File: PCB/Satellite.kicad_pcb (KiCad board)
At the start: 2 copper layers, 300 x 80 mm, 124 parts, among them SW1 SW_Push, SW10 SW_Push, SW11 SW_Push, SW12 SW_Push, SW13 SW_Push, SW14 SW_Push, SW15 SW_Push, SW16 SW_Push, SW17 SW_Push, SW18 SW_Push, SW19 SW_Push, SW2 SW_Push, SW20 SW_Push, SW21 SW_Push, SW22 SW_Push, SW23 SW_Push, SW24 SW_Push, SW25 SW_Push, SW26 SW_Push, SW27 SW_Push, SW28 SW_Push, SW29 SW_Push, SW3 SW_Push, SW30 SW_Push, SW31 SW_Push, SW32 SW_Push, SW33 SW_Push, SW34 SW_Push, SW35 SW_Push, SW36 SW_Push, SW37 SW_Push, SW38 SW_Push, SW39 SW_Push, SW4 SW_Push, SW40 SW_Push, SW41 SW_Push, SW42 SW_Push, SW43 SW_Push, SW44 SW_Push, SW45 SW_Push, SW46 SW_Push, SW47 SW_Push, SW48 SW_Push, SW5 SW_Push, SW6 SW_Push, SW7 SW_Push, SW8 SW_Push, SW9 SW_Push, Y1 16Mhz

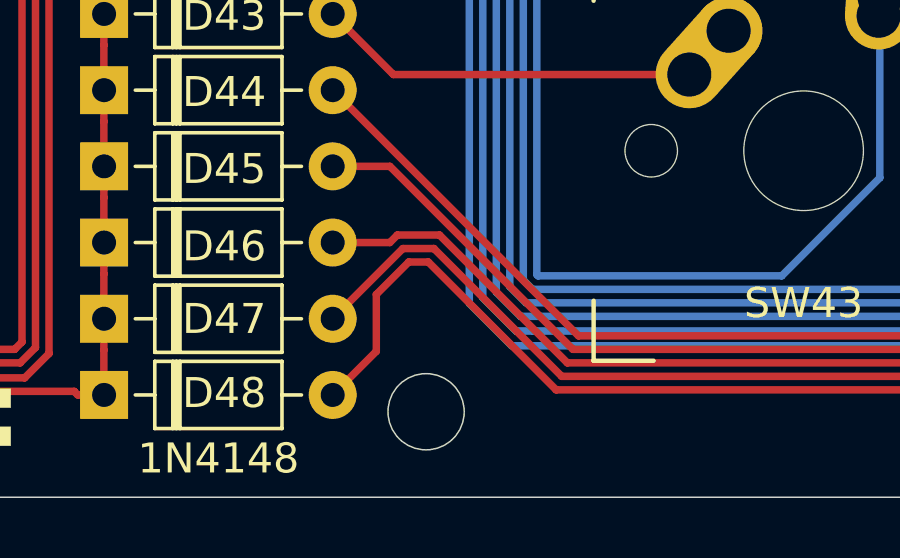
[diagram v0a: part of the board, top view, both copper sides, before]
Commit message: minor
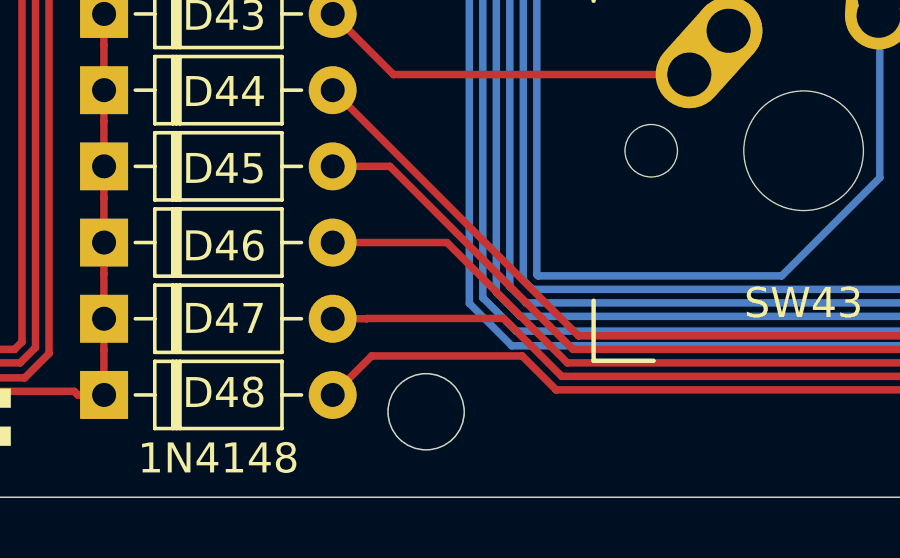
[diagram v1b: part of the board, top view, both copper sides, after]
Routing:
- net Net-(D48-Pad2): track 127.7 -> 124.0 mm
- net Net-(D47-Pad2): track 100.2 -> 98.2 mm
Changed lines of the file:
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@@
     (thickness 1.6)
     (drawings 28)
-    (tracks 936)
+    (tracks 934)
     (zones 0)
     (modules 124)
@@
   (segment (start 269.384018 101.479978) (end 269.38402 101.47998) (width 0.25) (layer F.Cu) (net 54))
   (segment (start 209.44716 101.479978) (end 269.384018 101.479978) (width 0.25) (layer F.Cu) (net 54))
-  (segment (start 205.187172 97.21999) (end 203.7796 97.21999) (width 0.25) (layer F.Cu) (net 54))
-  (segment (start 209.44716 101.479978) (end 205.187172 97.21999) (width 0.25) (layer F.Cu) (net 54))
-  (segment (start 203.52959 97.47) (end 201.626 97.47) (width 0.25) (layer F.Cu) (net 54))
-  (segment (start 203.7796 97.21999) (end 203.52959 97.47) (width 0.25) (layer F.Cu) (net 54))
+  (segment (start 205.43718 97.47) (end 209.44716 101.479978) (width 0.25) (layer F.Cu) (net 54))
+  (segment (start 201.626 97.47) (end 205.43718 97.47) (width 0.25) (layer F.Cu) (net 54))
   (segment (start 289.718 100.67598) (end 289.718 91.87) (width 0.25) (layer F.Cu) (net 55))
   (segment (start 288.46399 101.92999) (end 289.718 100.67598) (width 0.25) (layer F.Cu) (net 55))
-  (segment (start 201.626 100.01) (end 203.966 97.67) (width 0.25) (layer F.Cu) (net 55))
-  (segment (start 203.966 97.67) (end 205.000771 97.67) (width 0.25) (layer F.Cu) (net 55))
-  (segment (start 205.000771 97.67) (end 205.000771 97.670771) (width 0.25) (layer F.Cu) (net 55))
   (segment (start 288.463988 101.929988) (end 288.46399 101.92999) (width 0.25) (layer F.Cu) (net 55))
   (segment (start 209.259988 101.929988) (end 288.463988 101.929988) (width 0.25) (layer F.Cu) (net 55))
-  (segment (start 205.000771 97.670771) (end 209.259988 101.929988) (width 0.25) (layer F.Cu) (net 55))
+  (segment (start 202.75737 100.01) (end 202.76737 100) (width 0.25) (layer F.Cu) (net 55))
+  (segment (start 201.626 100.01) (end 202.75737 100.01) (width 0.25) (layer F.Cu) (net 55))
+  (segment (start 207.33 100) (end 209.259988 101.929988) (width 0.25) (layer F.Cu) (net 55))
+  (segment (start 202.76737 100) (end 207.33 100) (width 0.25) (layer F.Cu) (net 55))
   (segment (start 308.768 100.996) (end 308.768 91.87) (width 0.25) (layer F.Cu) (net 56))
   (segment (start 301.267002 102.38) (end 301.277002 102.39) (width 0.25) (layer F.Cu) (net 56))
   (segment (start 301.277002 102.39) (end 307.374 102.39) (width 0.25) (layer F.Cu) (net 56))
   (segment (start 307.374 102.39) (end 308.768 100.996) (width 0.25) (layer F.Cu) (net 56))
-  (segment (start 201.626 102.55) (end 203.08 101.096) (width 0.25) (layer F.Cu) (net 56))
-  (segment (start 203.08 99.2) (end 204.15999 98.12001) (width 0.25) (layer F.Cu) (net 56))
-  (segment (start 203.08 101.096) (end 203.08 99.2) (width 0.25) (layer F.Cu) (net 56))
-  (segment (start 204.15999 98.12001) (end 204.8136 98.12001) (width 0.25) (layer F.Cu) (net 56))
-  (segment (start 204.8136 98.12001) (end 209.07359 102.38) (width 0.25) (layer F.Cu) (net 56))
   (segment (start 307.364 102.38) (end 307.374 102.39) (width 0.25) (layer F.Cu) (net 56))
   (segment (start 209.07359 102.38) (end 307.364 102.38) (width 0.25) (layer F.Cu) (net 56))
+  (segment (start 209.07359 102.379998) (end 209.073587 102.379997) (width 0.25) (layer F.Cu) (net 56))
+  (segment (start 209.07359 102.38) (end 209.07359 102.379998) (width 0.25) (layer F.Cu) (net 56))
+  (segment (start 209.073587 102.379997) (end 207.94359 101.25) (width 0.25) (layer F.Cu) (net 56))
+  (segment (start 202.926 101.25) (end 201.626 102.55) (width 0.25) (layer F.Cu) (net 56))
+  (segment (start 207.94359 101.25) (end 202.926 101.25) (width 0.25) (layer F.Cu) (net 56))
   (segment (start 185.262 36.655) (end 186.312 36.655) (width 0.25) (layer F.Cu) (net 57))
   (segment (start 183.887 35.28) (end 185.262 36.655) (width 0.25) (layer F.Cu) (net 57))
@@
   (segment (start 208.3 100.42) (end 208.33999 100.38001) (width 0.25) (layer B.Cu) (net 73))
   (segment (start 176.863946 86.319) (end 175.410444 86.319) (width 0.25) (layer B.Cu) (net 73))
-  (segment (start 207.74078 100.42) (end 206.62997 99.30919) (width 0.25) (layer B.Cu) (net 73))
   (segment (start 208.3 100.42) (end 207.74078 100.42) (width 0.25) (layer B.Cu) (net 73))
   (segment (start 206.62997 99.30919) (end 206.62997 88.45997) (width 0.25) (layer B.Cu) (net 73))
@@
   (segment (start 169.250445 62.333999) (end 166.730443 62.333999) (width 0.25) (layer B.Cu) (net 73))
   (segment (start 166.27 65.41359) (end 164.60359 67.08) (width 0.25) (layer B.Cu) (net 73))
+  (segment (start 207.74078 100.42) (end 206.62997 99.30919) (width 0.25) (layer B.Cu) (net 73))
   (segment (start 315.114 33.735634) (end 315.114 51.23) (width 0.25) (layer B.Cu) (net 74))
   (segment (start 315.114 32.18) (end 315.114 33.735634) (width 0.25) (layer B.Cu) (net 74))
